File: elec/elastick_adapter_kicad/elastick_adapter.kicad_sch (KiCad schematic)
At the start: 12 parts, among them J2 DE9_Pins_MountingHoles

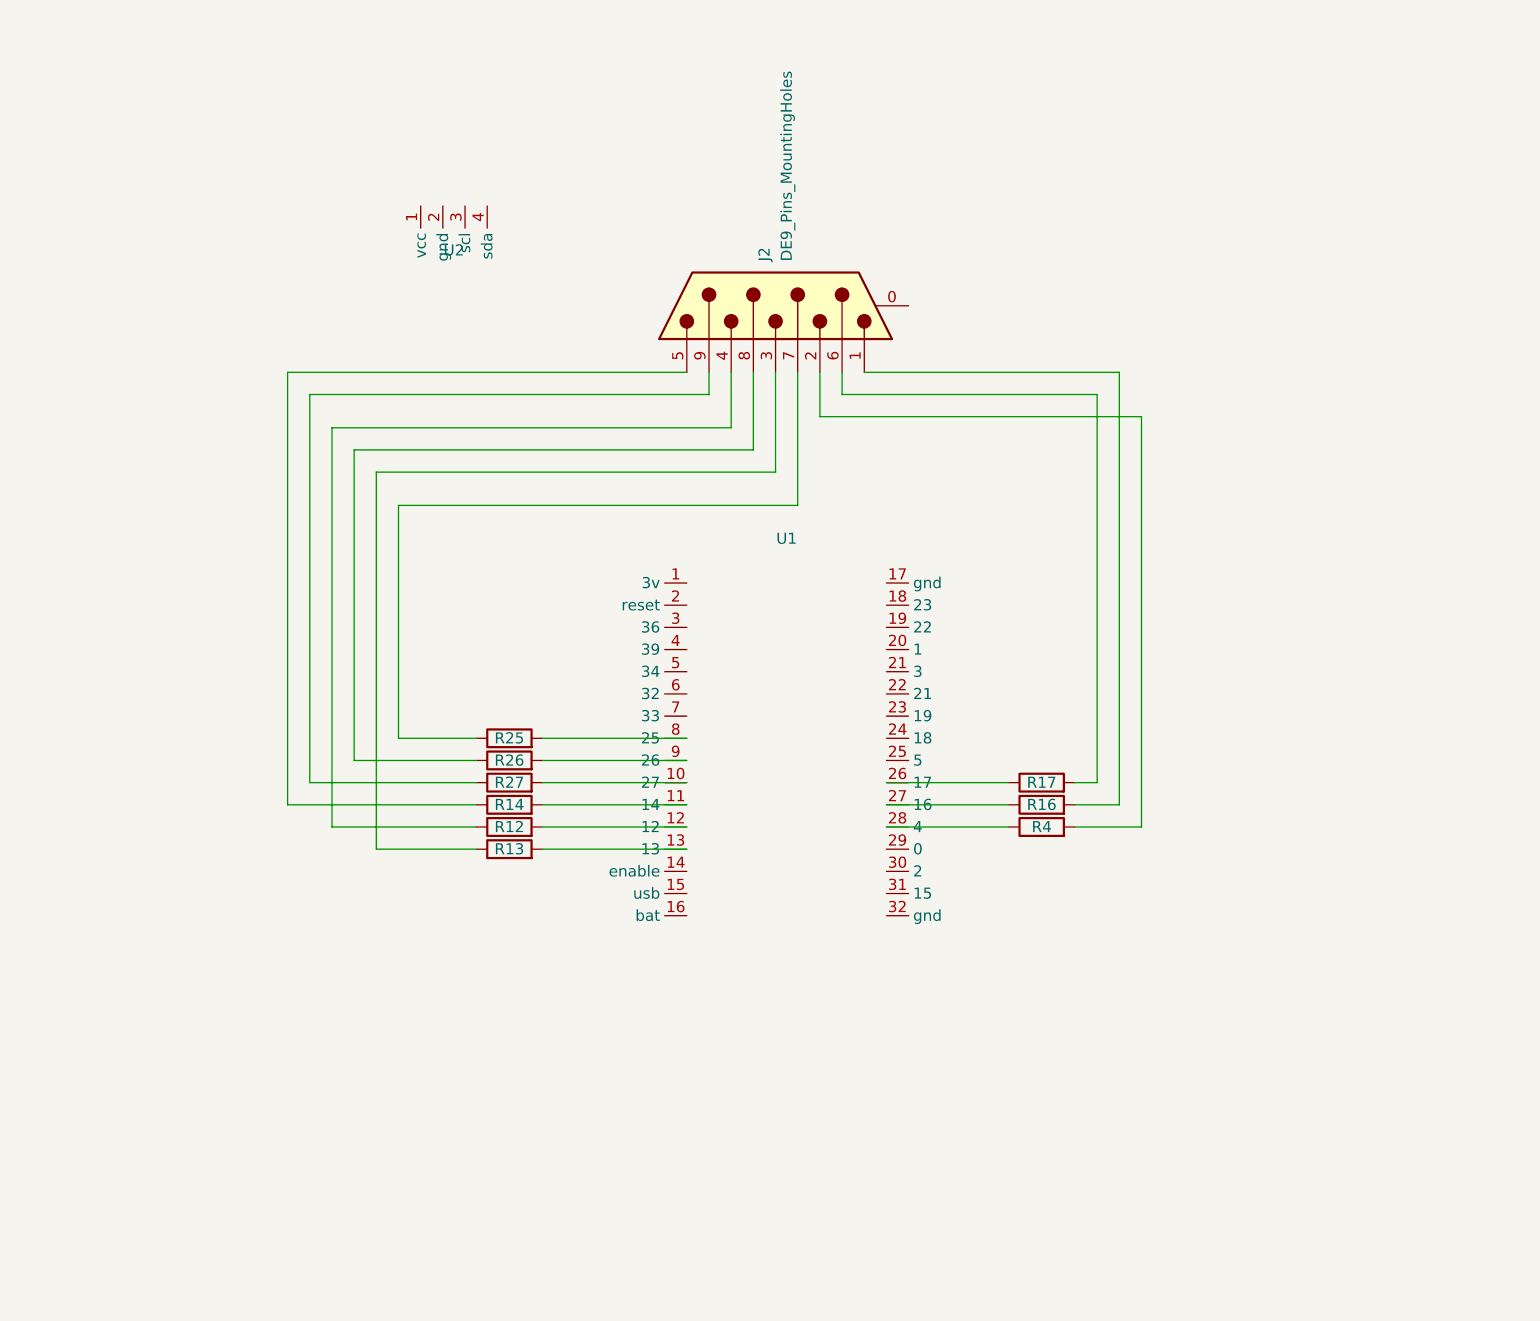
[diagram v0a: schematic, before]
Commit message: update kicad
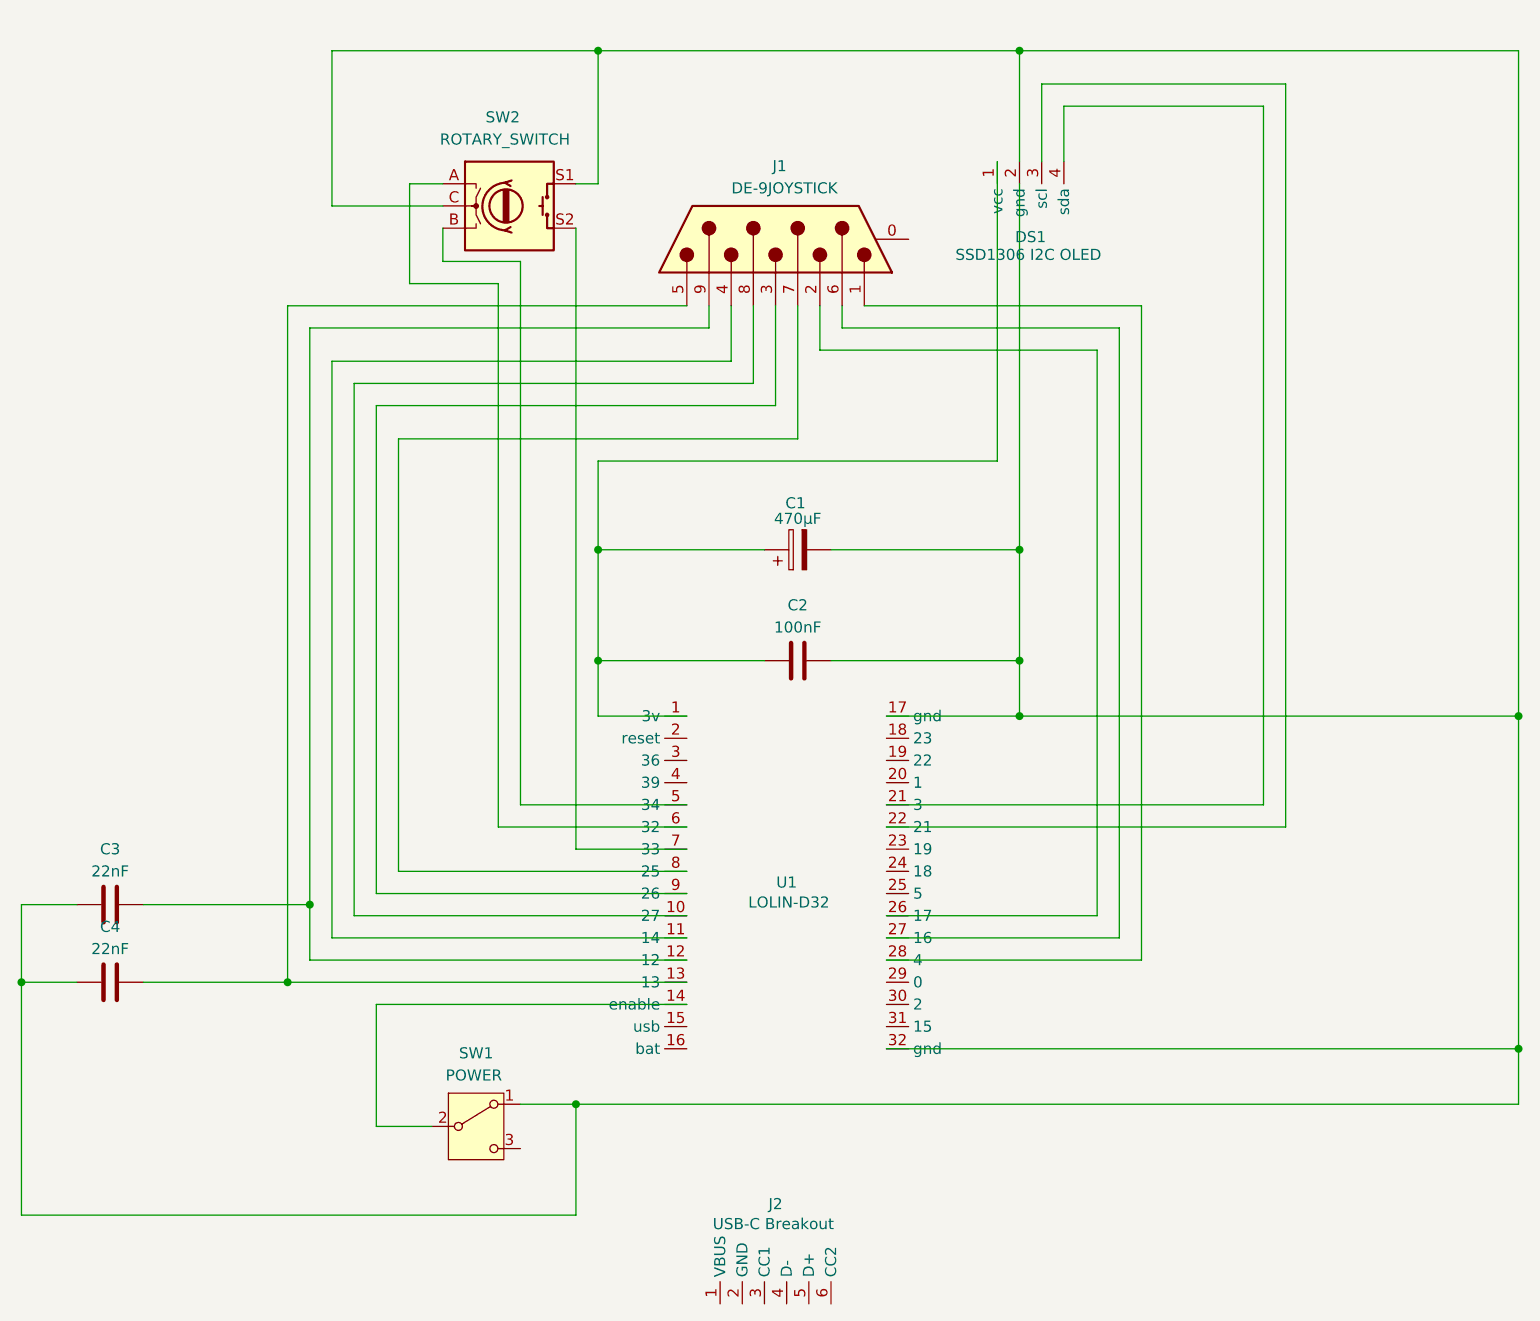
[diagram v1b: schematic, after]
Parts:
- removed R12, R13, R14, R16, R17, R25, R26, R27, R4: 330, Resistor_THT:R_Axial_DIN0207_L6.3mm_D2.5mm_P7.62mm_Horizontal, symbol Device:R
- added C1: 470µF, Capacitor_THT:CP_Radial_D8.0mm_P3.50mm, symbol Device:C_Polarized
- added C2: 100nF, Capacitor_THT:C_Disc_D5.0mm_W2.5mm_P5.00mm, symbol Device:C
- added C3, C4: 22nF, Capacitor_THT:C_Disc_D5.0mm_W2.5mm_P5.00mm, symbol Device:C
- added J2: USB-C Breakout, elastick:usbc, symbol elastick:usbc
- added SW1: POWER, Button_Switch_THT:SW_Slide_SPDT_Angled_CK_OS102011MA1Q, symbol Switch:SW_SPDT
- added SW2: ROTARY_SWITCH, Rotary_Encoder:RotaryEncoder_Alps_EC11E-Switch_Vertical_H20mm, symbol Device:RotaryEncoder_Switch
- DS1: renamed from U2; value ~ -> SSD1306 I2C OLED
- J1: renamed from J2; value DE9_Pins_MountingHoles -> DE-9JOYSTICK
- U1: value ~ -> LOLIN-D32
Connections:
- net at J1.3: now also U1.9 (26)
- net at U1.13: now also J1.5, C4.2
- net at J1.7: now also U1.8 (25)
- net at U1.11 (14): now also J1.4
- net at U1.12: now also J1.9, C3.2
- net at DS1.1 (vcc): now also U1.1 (3v), C1.1, C2.1
- net at DS1.2 (gnd): now also U1.17 (gnd), U1.32 (gnd), C1.2, C2.2, C3.1, C4.1, SW1.1 (A), SW2.C, SW2.S1
- net at DS1.3 (scl): now also U1.22 (21)
- net at DS1.4 (sda): now also U1.21 (3)
- net at U1.10 (27): now also J1.8
- net at U1.14 (enable): now also SW1.2 (B)
- net at U1.26 (17): now also J1.2
- net at U1.27 (16): now also J1.6
- net at U1.28 (4): now also J1.1
- net at U1.5 (34): now also SW2.B
- net at U1.6 (32): now also SW2.A
- net at U1.7 (33): now also SW2.S2
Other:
- moved on the sheet: DS1, J1, U1
